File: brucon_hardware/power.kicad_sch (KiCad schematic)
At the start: 27 parts, among them J201 WTB01W03BB, Q201 AO3400A, SW201 AA04A02010000018A, U201 TP4056, U202 MT3608L, U203 HT75xx-1-SOT89

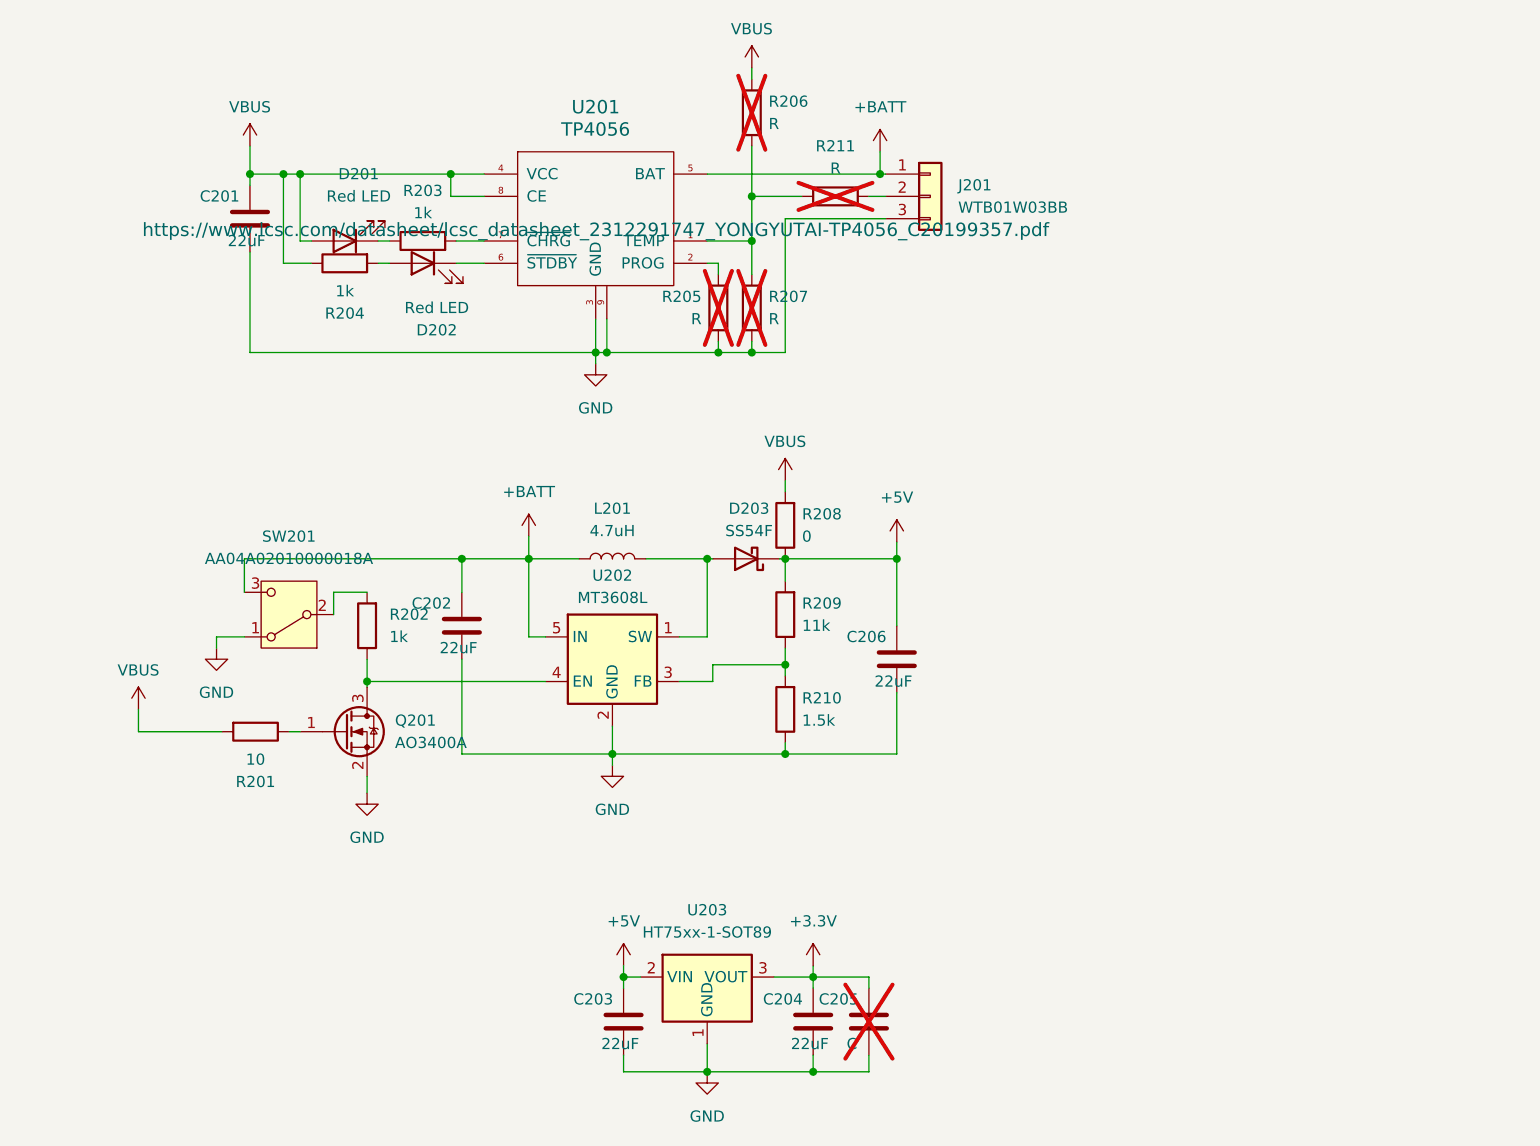
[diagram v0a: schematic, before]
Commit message: Updated hardware
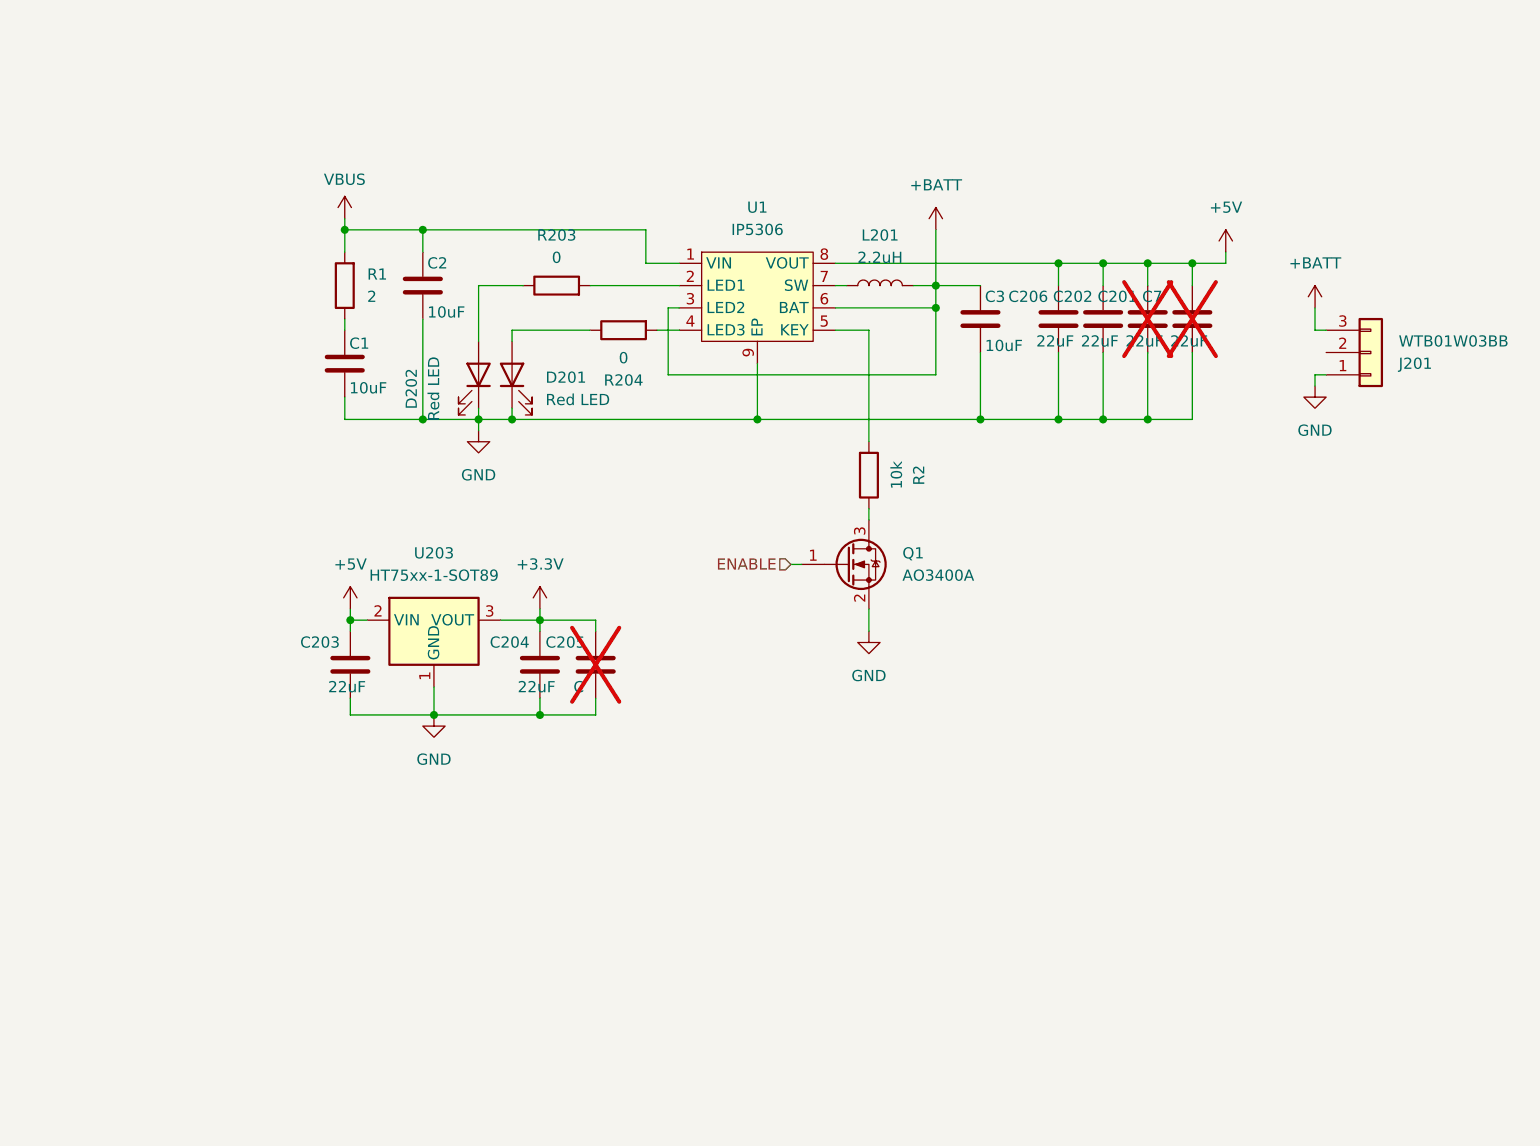
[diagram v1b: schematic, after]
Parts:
- removed D203: SS54F, Diode_SMD:D_SMA, symbol Device:D_Schottky
- removed Q201: AO3400A, Package_TO_SOT_SMD:SOT-23, symbol Transistor_FET:AO3400A
- removed R201: 10, Resistor_SMD:R_0402_1005Metric, symbol Device:R
- removed R202: 1k, Resistor_SMD:R_0402_1005Metric, symbol Device:R
- removed R205, R206, R207, R211: R, Resistor_SMD:R_0402_1005Metric, symbol Device:R
- removed R208: 0, Resistor_SMD:R_0402_1005Metric, symbol Device:R
- removed R209: 11k, Resistor_SMD:R_0402_1005Metric, symbol Device:R
- removed R210: 1.5k, Resistor_SMD:R_0402_1005Metric, symbol Device:R
- removed SW201: AA04A02010000018A, Button_Switch_SMD:SW_SPDT_PCM12, symbol Switch:SW_SPDT
- removed U201: TP4056, Package_SO:SOP-8-1EP_4.57x4.57mm_P1.27mm_EP4.57x4.45mm, symbol tp4056:TP4056
- removed U202: MT3608L, Package_TO_SOT_SMD:SOT-23-6, symbol Regulator_Switching:MT3608
- added C1, C2, C3: 10uF, Capacitor_SMD:C_0603_1608Metric, symbol Device:C
- added C7: 22uF, Capacitor_SMD:C_0805_2012Metric, symbol Device:C
- added Q1: AO3400A, Package_TO_SOT_SMD:SOT-23, symbol Transistor_FET:AO3400A
- added R1: 2, Resistor_SMD:R_0402_1005Metric, symbol Device:R
- added R2: 10k, Resistor_SMD:R_0402_1005Metric, symbol Device:R
- added U1: IP5306, Package_SO:HSOP-8-1EP_3.9x4.9mm_P1.27mm_EP2.41x3.1mm_ThermalVias, symbol IP5306:IP5306
- C201: now not fitted
- L201: value 4.7uH -> 2.2uH; footprint Inductor_SMD:L_Sunlord_MWSA0603S -> Inductor_SMD:L_Changjiang_FNR5030S; LCSC C5307631 -> C7588710; PNR XR0630-4R7M -> (none)
- R203, R204: value 1k -> 0; LCSC C21190 -> (none)
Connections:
- net +5V: now also C201.1, C202.1, C7.1, U1.8 (VOUT)
- net +BATT: now also J201.3 (Pin_3), L201.2, C3.1, U1.3 (LED2), U1.6 (BAT); no longer C202.1, J201.1 (Pin_1), L201.1
- net GND: now also D201.1 (K), D202.1 (K), J201.1 (Pin_1), C1.2, C2.2, C3.2, C7.2, Q1.2 (S), U1.9 (EP); no longer J201.3 (Pin_3)
- net VBUS: now also C2.1, R1.2, U1.1 (VIN); no longer C201.1, D201.2 (A), R204.1
- net at R204.2: now also U1.4 (LED3); no longer D202.2 (A)
- net at R203.1: now also D202.2 (A); no longer D201.1 (K)
- net at R203.2: now also U1.2 (LED1)
- new net: D201.2 (A), R204.1
- new net: R2.2, U1.5 (KEY)
- new net: L201.1, U1.7 (SW)
- new net: Q1.3 (D), R2.1
- new net: C1.1, R1.1
- new net ENABLE: Q1.1 (G)
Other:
- moved on the sheet: C202, C203, C204, C205, C206, D201, D202, J201, L201, R203, R204, U203
